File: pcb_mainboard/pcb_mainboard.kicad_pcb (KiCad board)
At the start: 2 copper layers, 47 x 59.7 mm, 11 parts, among them J1 Ringer Module, J2 Phone Body, Q1 Q_NMOS_GSD, Q2 Q_NMOS_GSD, U1 Adafruit_Audio_FX_+_Amp

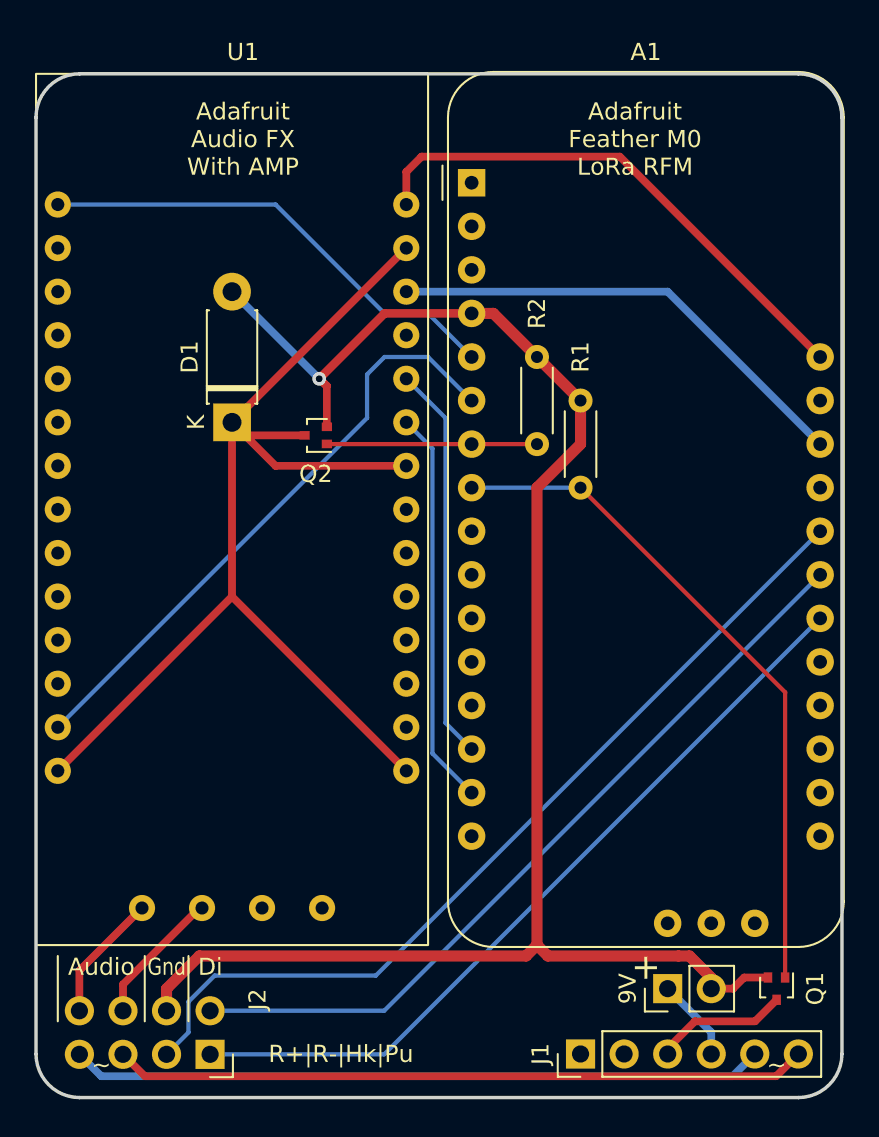
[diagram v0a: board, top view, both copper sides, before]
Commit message: V1 board as sent to oshpark
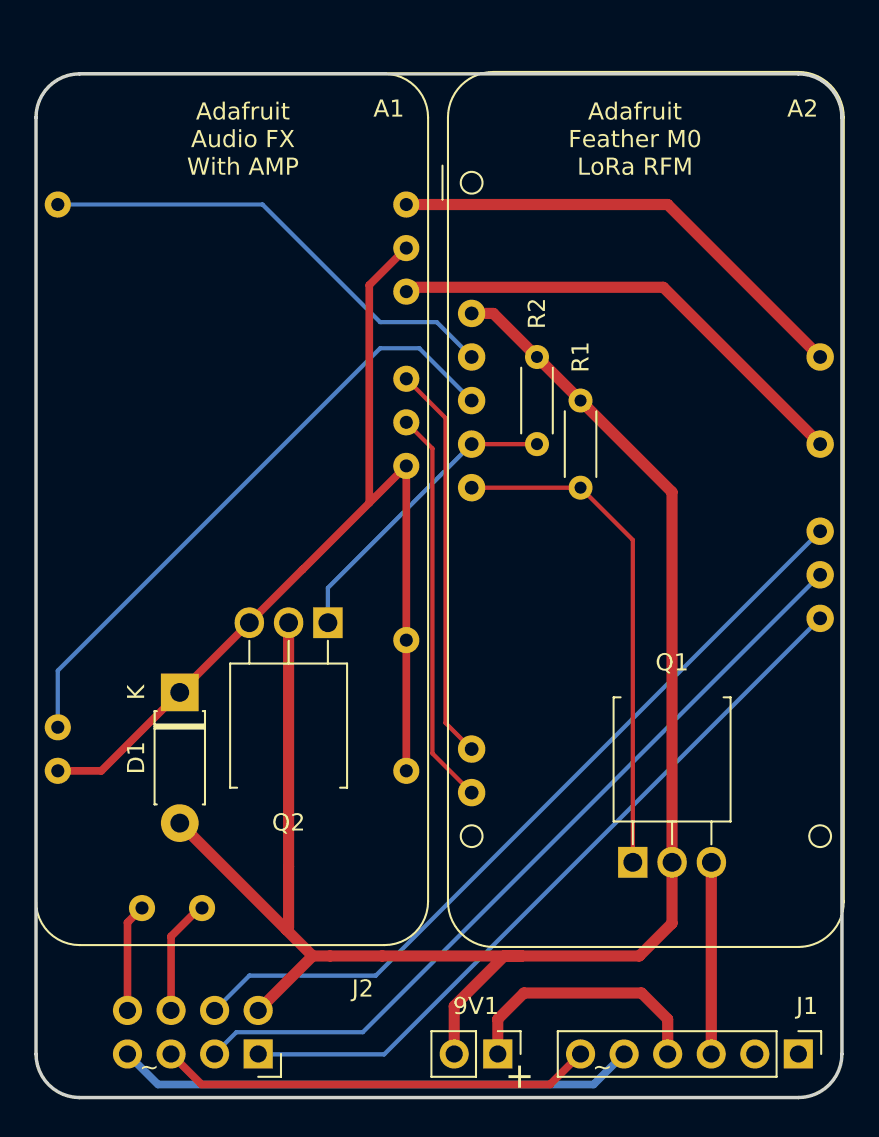
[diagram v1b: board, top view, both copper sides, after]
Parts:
- added G***: LOGO, LOGO, F.Cu at (104.1, 81.3)
- Q1, Q2: footprint Package_TO_SOT_SMD:SOT-416 -> Package_TO_SOT_THT:TO-251-3-1EP_Horizontal_TabDown
- moved D1 16.0 mm to (77.0, 105.9), turned to -90 degrees
- moved J1 12.7 mm to (113.0, 127.0), turned to -90 degrees
- moved Q1 11.2 mm to (103.4, 115.8), turned to 0 degrees
- moved Q2 10.9 mm to (85.6, 101.9)
- moved 9V1 10.6 mm to (95.5, 127.0), turned to -90 degrees
- moved G*** 3.06 mm to (89.9, 97.8)
- moved J2 2.80 mm to (81.5, 127.0)
- renumbered 9V to 9V1, U1 to A1, A1 to A2
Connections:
- J2 pad 2: SW_DIAL -> GND
- J2 pad 3: SW_HOOK -> SW_DIAL
- J2 pad 4: GND -> SW_HOOK
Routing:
- net /Ringer AC A: track 40.4 -> 25.3 mm
- net RGATE: track 39.9 -> 29.5 mm
- net /9V Pow: track 4.86 -> 15.2 mm
- net /Ringer AC B: track 40.5 -> 30.4 mm
- net /Audio GND: track 69.0 -> 61.2 mm
- net AGATE: track 12.4 -> 17.7 mm
- net SW_HOOK: track 51.8 -> 46.9 mm
- net /Audio Vin: track 31.2 -> 27.8 mm
- net /Ringer GND: track 7.84 -> 11.2 mm
- net GND: track 101.6 -> 104.6 mm, vias 1 -> 0
- net SW_DIAL_PULSE: track 46.1 -> 43.3 mm
- net /Audio L+: track 7.50 -> 6.32 mm
- net /Audio L-: track 7.99 -> 6.81 mm
- net AAct: track 35.6 -> 36.5 mm
- net SW_DIAL: track 46.1 -> 46.9 mm
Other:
- board text added: "github.com/jonmon6691 /arduino_longdistance"
- board text removed: "Audio"
- board text removed: "Di"
- board text removed: "Gnd"
- board text removed: "R+|R-|Hk|Pu"
